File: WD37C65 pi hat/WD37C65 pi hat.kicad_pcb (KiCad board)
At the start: 2 copper layers, 64 x 55 mm, 44 parts, among them CN1 FLOPPY CONNECTOR, J1 /DCHG, J10 ftdi power, J11 CTS, J12 DTR, J14 Raspberry_Pi_2_3, J15 GPIO10, J16 GPIO9, J17 Barrel_Jack_Switch, J2 /HDL, J3 MO1, J4 MO2, J5 DS1, J6 DS2, J7 serial, J8 i2c, J9 DCHGEN, Q1 16.000, U1 WD37C65

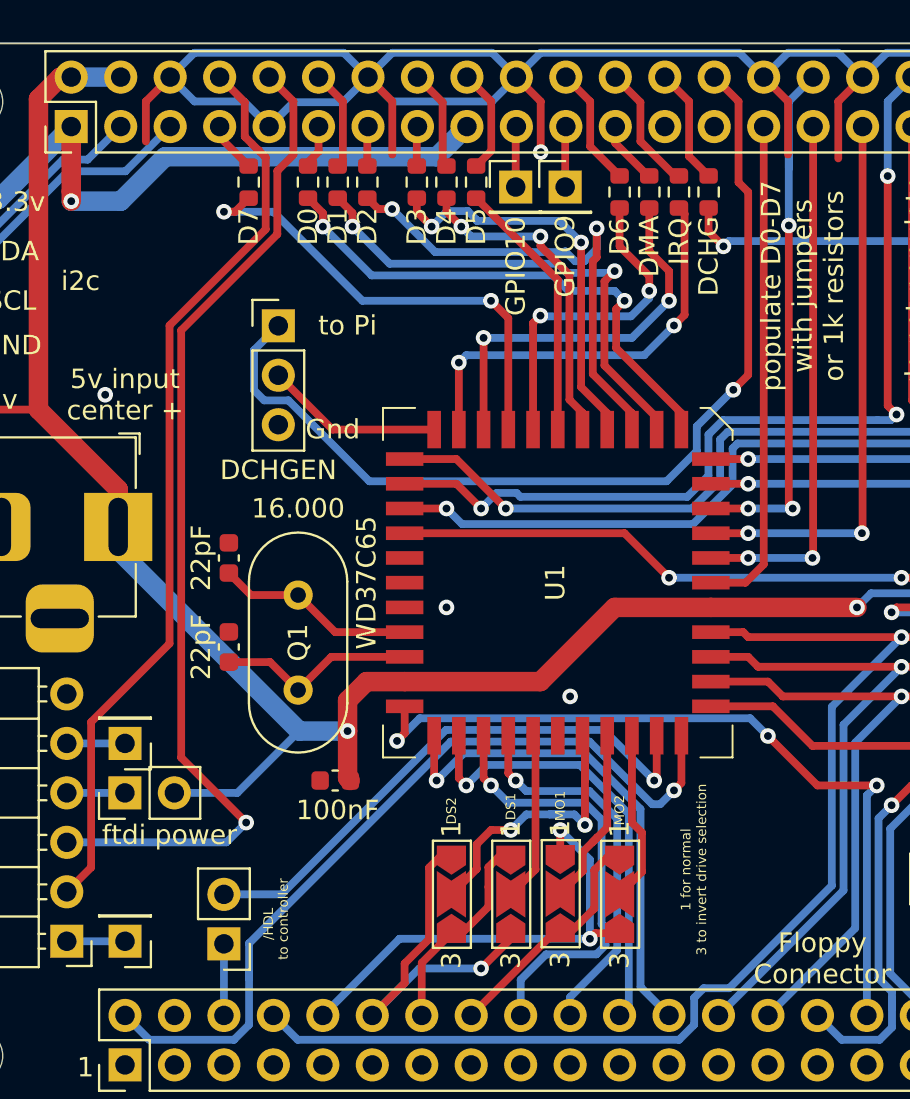
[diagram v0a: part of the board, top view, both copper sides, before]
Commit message: added gerbers, ERC DRC fixes
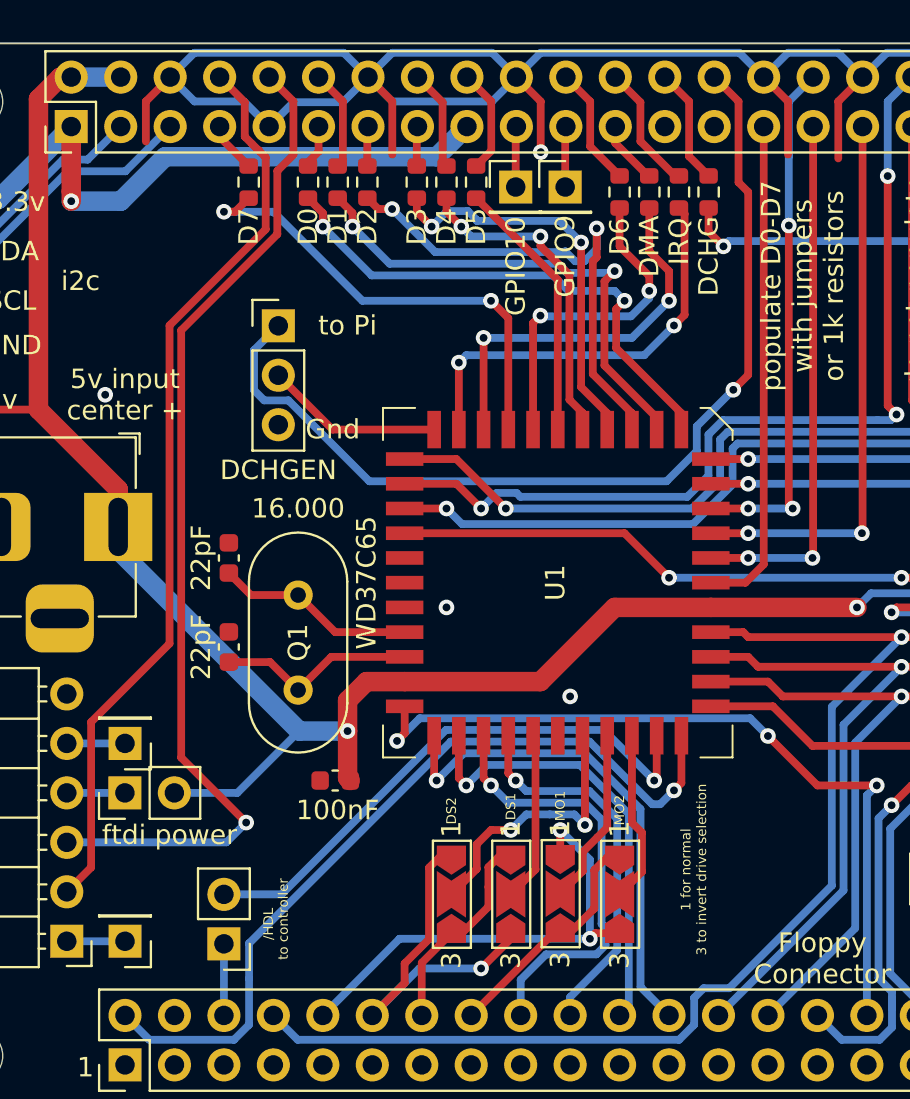
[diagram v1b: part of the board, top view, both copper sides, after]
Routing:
- net *DS2: track 15.7 -> 14.2 mm
- net *MO1: track 10.2 -> 9.11 mm
- net A0: track 27.6 -> 27.0 mm
